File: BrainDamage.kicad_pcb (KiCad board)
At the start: 2 copper layers, 100 x 100 mm, 51 parts, among them CON1 AVR-ISP-10, IC1 ATMEGA328P-A, J1 TEST_2P, J2 TEST_2P, J3 TEST_2P, J4 TEST_2P, J5 TEST_2P, J6 TEST_2P, J7 FTDI, J8 Bluetooth, P1 CONN_01X03, P10 CONN_01X03, P11 CONN_01X03, P12 CONN_01X03, P13 CONN_01X03, P14 CONN_01X03, P15 CONN_01X03, P16 CONN_01X03, P17 CONN_01X03, P2 CONN_01X03, P3 CONN_01X03, P4 CONN_01X03, P5 CONN_01X03, P6 CONN_01X03, P7 CONN_01X03, P8 CONN_01X08, P9 CONN_01X03, SW1 SW_PUSH, U1 PCA9685-TSSOP, X1 CRYSTAL_SMD

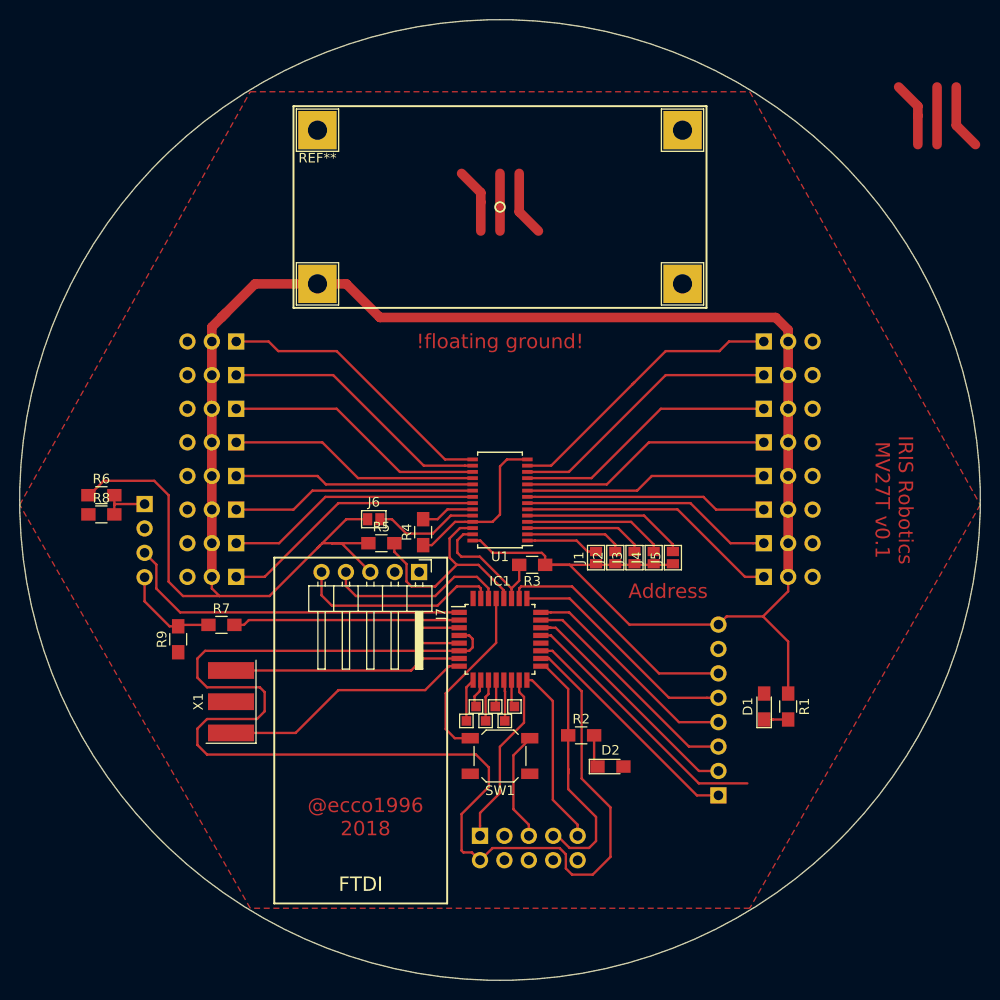
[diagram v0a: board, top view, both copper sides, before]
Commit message: Add files via upload
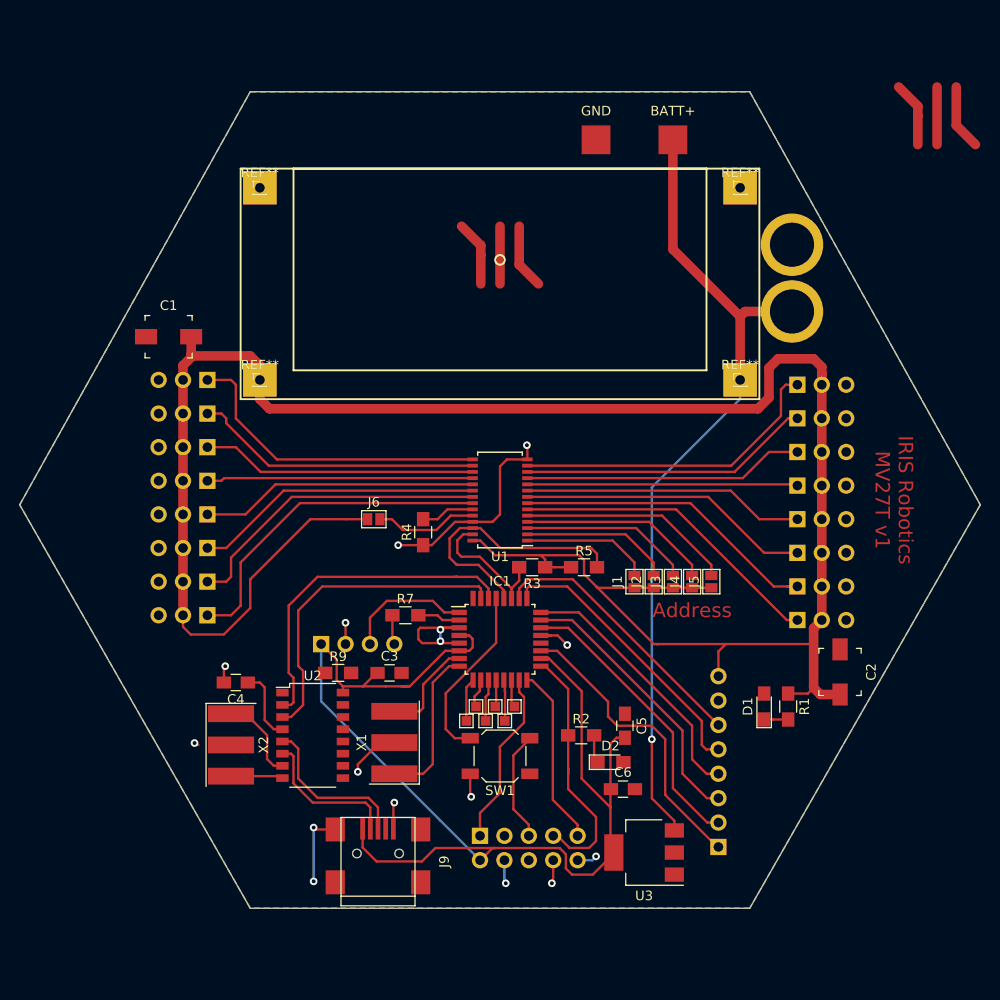
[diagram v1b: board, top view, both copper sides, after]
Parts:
- removed J7: FTDI, Pin_Headers:Pin_Header_Angled_1x05_Pitch2.54mm
- removed R6: 20K, Resistors_SMD:R_0805_HandSoldering
- removed R8: 10K, Resistors_SMD:R_0805_HandSoldering
- removed the REF** at (219.0, 25.0)
- removed the REF** at (181.0, 25.0)
- removed the REF** at (181.0, 41.0)
- removed the REF** at (219.0, 41.0)
- added BATT+: Measurement_Point_Square-SMD-Pad_Big, Measurement_Points:Measurement_Point_Square-SMD-Pad_Big, F.Cu at (218.0, 26.0)
- added C1: C, Capacitors_SMD:C_Trimmer_Murata_TZB4-A, F.Cu at (165.5, 46.5)
- added C2: C, Capacitors_SMD:C_Trimmer_Murata_TZB4-A, F.Cu at (235.4, 81.4)
- added C3: C, Capacitors_SMD:C_0805_HandSoldering, F.Cu at (188.5, 81.5)
- added C4: 1n, Capacitors_SMD:C_0805_HandSoldering, F.Cu at (172.5, 82.5)
- added C5: 1n, Capacitors_SMD:C_0805_HandSoldering, F.Cu at (213.0, 87.0)
- added C6: C, Capacitors_SMD:C_0805_HandSoldering, F.Cu at (212.8, 93.6)
- added GND: Measurement_Point_Square-SMD-Pad_Big, Measurement_Points:Measurement_Point_Square-SMD-Pad_Big, F.Cu at (210.0, 26.0)
- added J10: Conn_01x02, RC-Battery-Connectors:XT-60_male, B.Cu at (230.4, 40.4)
- added J9: USB_OTG, Connectors:USB_Mini-B, F.Cu at (187.3, 100.5)
- added REF**: Pin_Header_Straight_1x01_Pitch1.00mm, Pin_Headers:Pin_Header_Straight_1x01_Pitch1.00mm, F.Cu at (175.0, 31.0)
- added REF**: Pin_Header_Straight_1x01_Pitch1.00mm, Pin_Headers:Pin_Header_Straight_1x01_Pitch1.00mm, F.Cu at (225.0, 31.0)
- added REF**: Pin_Header_Straight_1x01_Pitch1.00mm, Pin_Headers:Pin_Header_Straight_1x01_Pitch1.00mm, F.Cu at (225.0, 51.0)
- added REF**: Pin_Header_Straight_1x01_Pitch1.00mm, Pin_Headers:Pin_Header_Straight_1x01_Pitch1.00mm, F.Cu at (175.0, 51.0)
- added U2: CH340G, Housings_SSOP:SOP-16_4.4x10.4mm_Pitch1.27mm, F.Cu at (180.5, 88.0)
- added U3: AP1117-50, TO_SOT_Packages_SMD:SOT-223-3Lead_TabPin2, F.Cu at (215.0, 100.2)
- added X2: CRYSTAL_SMD, Crystals:Resonator_SMD_muRata_SFSKA-3pin_7.9x3.8mm_HandSoldering, F.Cu at (172.0, 89.0)
- moved J8 23.5 mm to (181.4, 78.5), turned to 270 degrees
- moved R5 21.2 mm to (208.8, 70.5)
- moved R7 19.2 mm to (190.2, 75.5)
- moved X1 17.5 mm to (189.0, 88.8)
- moved R9 17.0 mm to (183.2, 81.5), turned to 0 degrees
- moved S0 5.70 mm to (231.0, 76.0)
- moved S1 5.70 mm to (231.0, 72.5)
- moved S2 5.70 mm to (231.0, 69.0)
- moved S3 5.70 mm to (231.0, 65.5)
- moved S4 5.70 mm to (231.0, 62.0)
- moved S5 5.70 mm to (231.0, 58.5)
- moved S6 5.70 mm to (231.0, 55.0)
- moved S7 5.70 mm to (231.0, 51.5)
- moved P8 5.37 mm to (222.7, 99.6)
- moved S10 5.00 mm to (169.5, 58.0)
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- renumbered P16 to S0, P14 to S1, P13 to S10, P12 to S11, P11 to S12, P10 to S13, P9 to S14, P7 to S15, P6 to S2, P5 to S3, P4 to S4, P3 to S5, P2 to S6, P1 to S7, P17 to S8, P15 to S9
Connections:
- J8 pad 1: Net-(J8-Pad1) -> +5V
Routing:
- net /BATT+: track 0.00 -> 85.2 mm, vias 0 -> 1
- net /TXB: track 36.8 -> 13.3 mm
- net /RXB: track 23.6 -> 4.46 mm
- net +5V: track 372.8 -> 354.1 mm
- net /RX: track 19.1 -> 35.4 mm
- net Net-(J9-Pad3): track 0.00 -> 16.0 mm
- net Net-(J9-Pad2): track 0.00 -> 14.5 mm
- net GND: track 56.0 -> 69.2 mm, vias 0 -> 15
- net /TX: track 21.4 -> 33.9 mm
- net /XTAL1: track 22.4 -> 10.5 mm
- net Net-(U2-Pad7): track 0.00 -> 9.06 mm
- net /XTAL2: track 24.9 -> 16.4 mm
- net Net-(C4-Pad1): track 0.00 -> 7.61 mm
- net /LED15: track 27.8 -> 35.1 mm
- net Net-(J8-Pad4): track 10.3 -> 3.08 mm
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- added copper zone on B.Cu, net GND
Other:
- board size 100 x 100 mm -> 100 x 85 mm
- board text added: "IRIS Robotics MV27T v1"
- board text removed: "!floating ground!"
- board text removed: "@ecco1996 2018"
- board text removed: "FTDI"
- board text removed: "IRIS Robotics MV27T v0.1"
